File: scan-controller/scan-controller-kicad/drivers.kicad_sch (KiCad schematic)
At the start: 50 parts, among them CN2 Motor, CN3 Fan, CN4 Lamp, Q1 CS12N06AE-G, U10 LGS5145, U11 MCP1416, U3 78L05, U4 DRV8871DDA, U6 TL431, U7 XL4015, U8 LM358

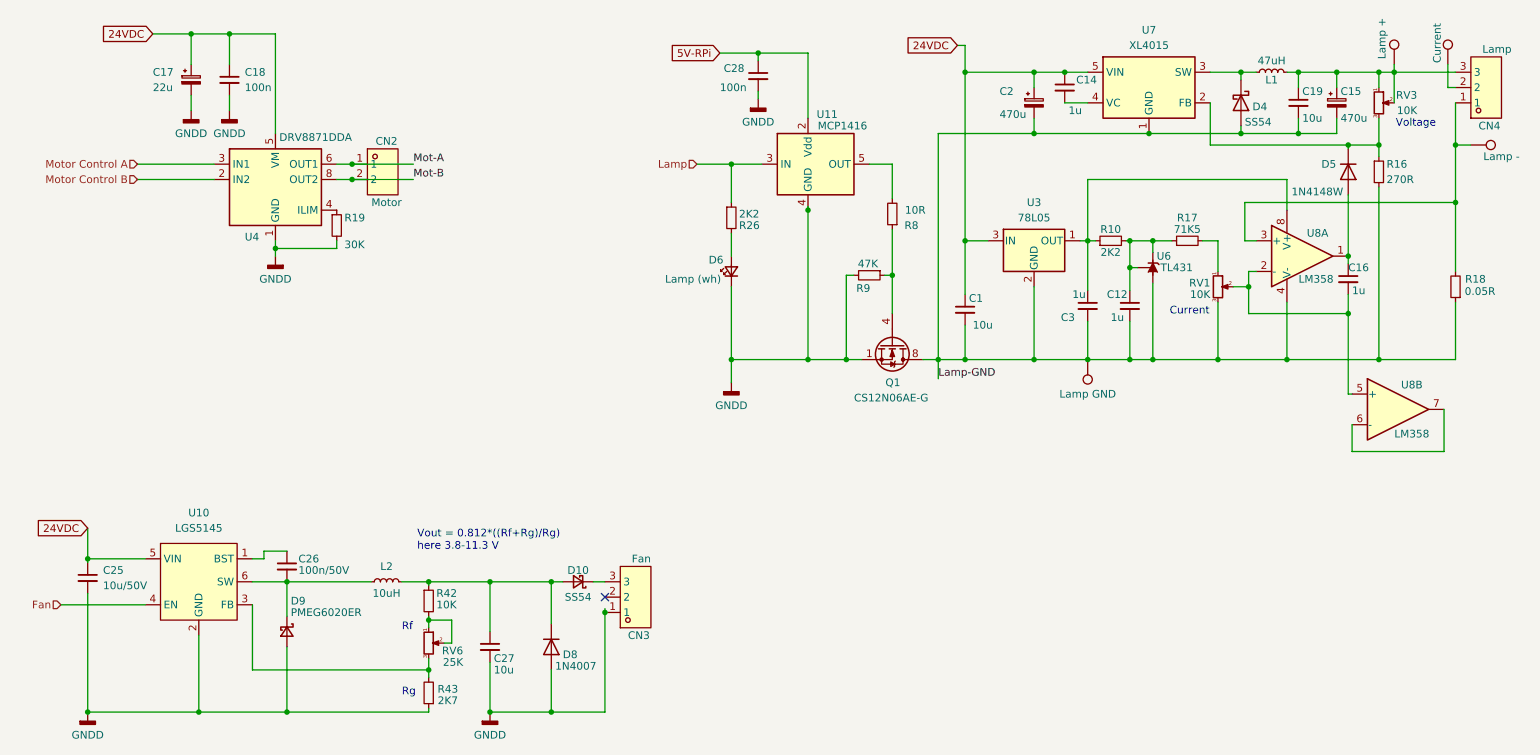
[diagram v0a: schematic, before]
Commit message: Cosmetic PCB Changes (not in sync with netlist yet)
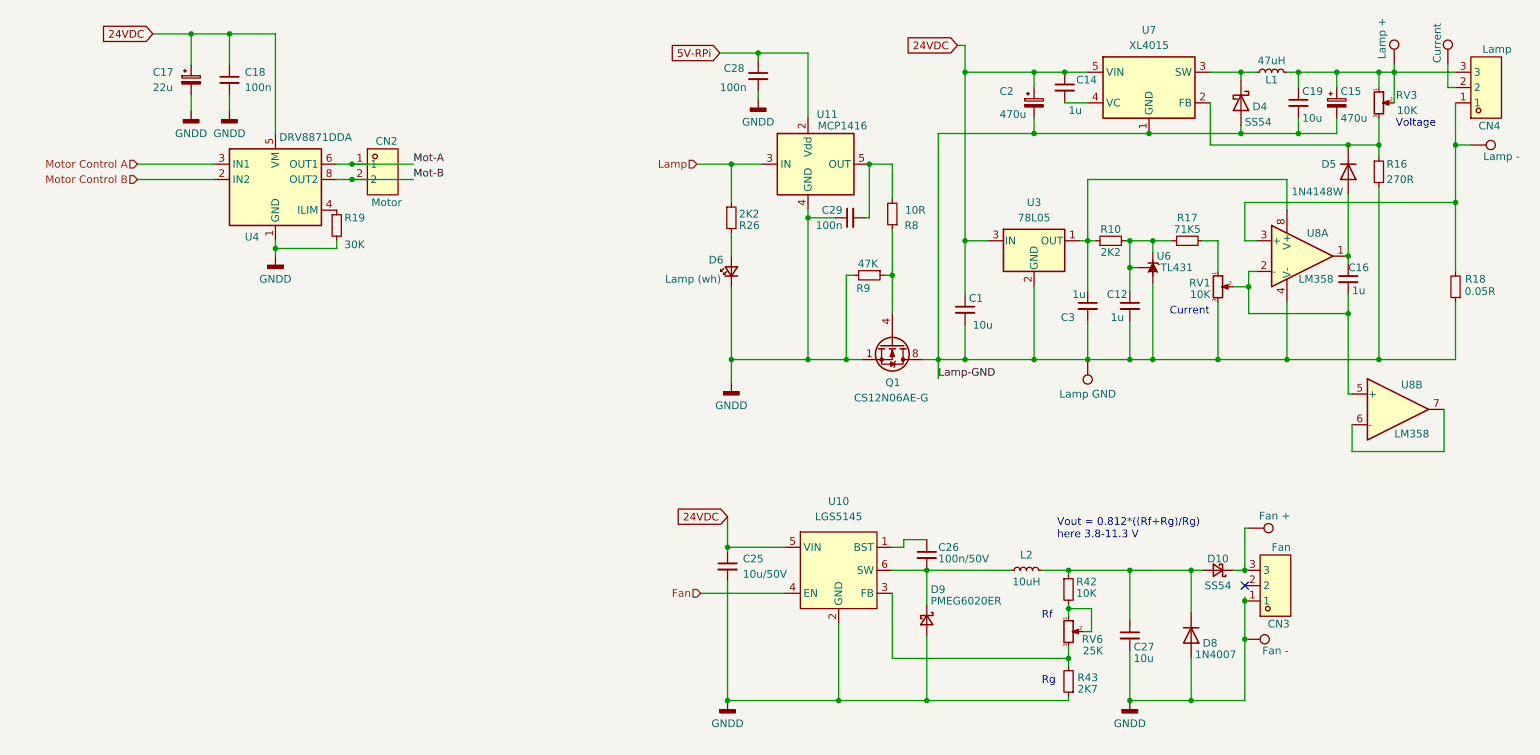
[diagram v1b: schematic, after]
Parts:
- added C29: 100n, Capacitor_SMD:C_0805_2012Metric, symbol Device:C_Small
- added TP17, TP18: TestPoint, Peacemans_Footprints:TestPoint_THTPad_1.5x1.5mm_Drill0.7mm_named, symbol Peacemans_Teile:TestPoint_named
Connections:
- net GNDD: now also C29.1, TP17.1
- net at R8.2, U11.5 (OUT): now also C29.2
- net at CN3.3, D10.1 (K): now also TP18.1
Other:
- moved on the sheet: C25, C26, C27, CN3, D10, D8, D9, L2, R42, R43, RV6, U10
